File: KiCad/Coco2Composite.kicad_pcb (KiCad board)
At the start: 2 copper layers, 52 x 36.5 mm, 19 parts, among them J1 MA03-1, J2 MA05-1, J3 AUDIO_JACK_3.5MM_PTH, Q1 PN2907, Q2 2N2222, U1 MC1372

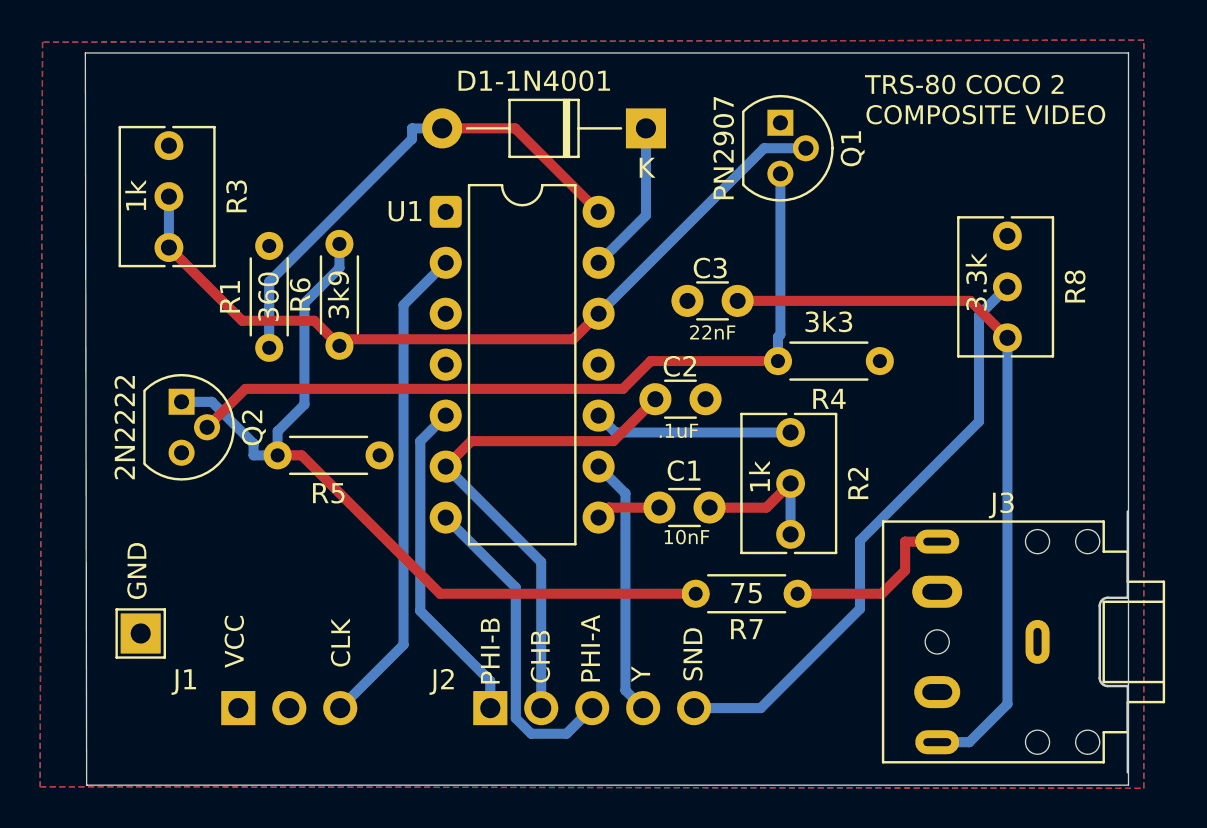
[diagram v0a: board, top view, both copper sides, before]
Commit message: updated layout, shifted headers a tiny bit
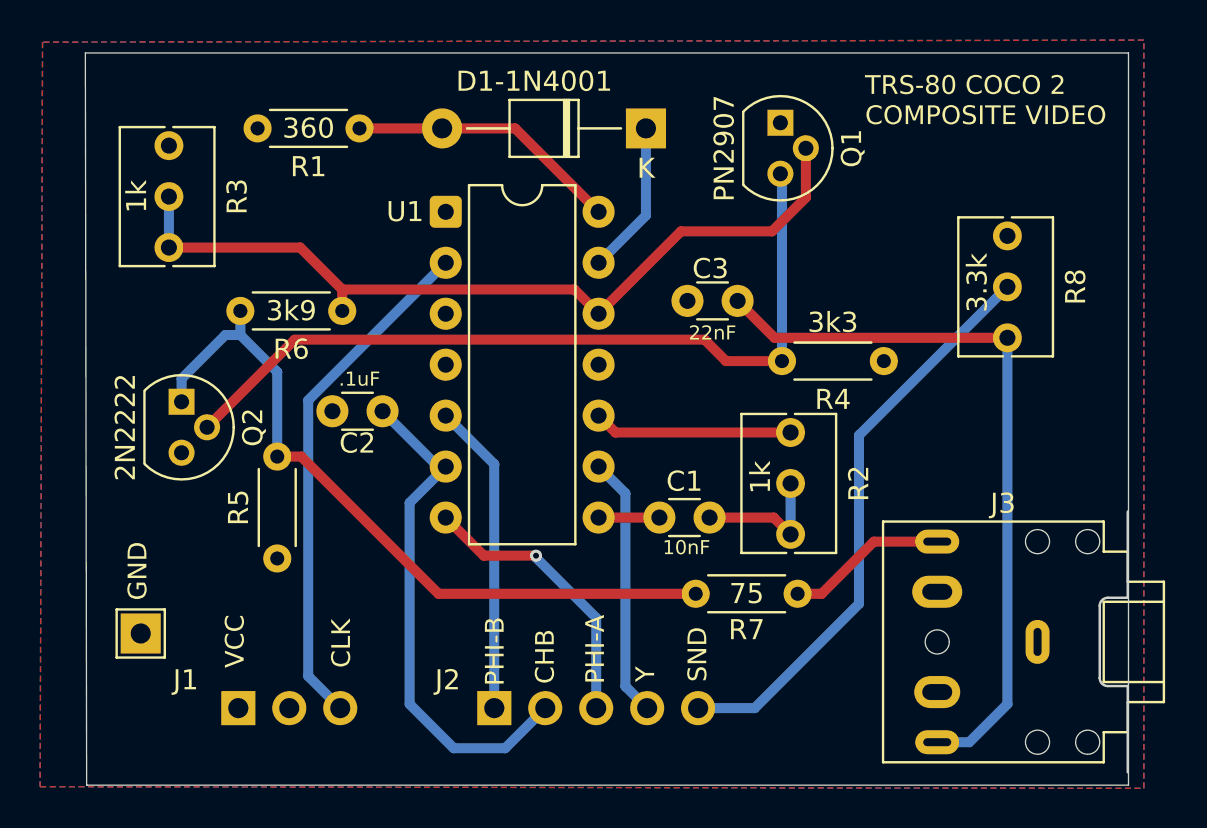
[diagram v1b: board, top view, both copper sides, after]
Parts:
- moved C2 13.6 mm to (130.8, 106.2), turned to 180 degrees
- moved R1 11.8 mm to (129.7, 92.1), turned to 180 degrees
- moved R5 7.24 mm to (125.6, 113.5), turned to 90 degrees
- moved R6 1.75 mm to (128.8, 101.2), turned to 180 degrees
- moved C1 0.50 mm to (144.7, 111.5)
- moved R4 0.20 mm to (155.8, 103.7)
- moved J2 0.20 mm to (136.4, 121.0)
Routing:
- net Net-(U1-RF_TANK_2): track 24.9 -> 13.6 mm
- net Net-(Q2-E): track 41.8 -> 36.7 mm
- net Net-(U1-COL_A_IN): track 16.1 -> 14.1 mm, vias 0 -> 1
- net Net-(U1-OSC_IN): track 24.4 -> 25.7 mm
- net Net-(U1-RF_OUT): track 40.4 -> 41.6 mm
- net Net-(Q2-B): track 39.2 -> 40.3 mm
- net Net-(U1-COL_B_IN): track 16.6 -> 15.6 mm
- net COMP_OUT: track 8.88 -> 8.04 mm
